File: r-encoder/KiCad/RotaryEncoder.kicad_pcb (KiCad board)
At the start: 2 copper layers, 39 x 39 mm, 15 parts, among them J1 Conn_01x06, U1 PEC11R-4325F-S0012

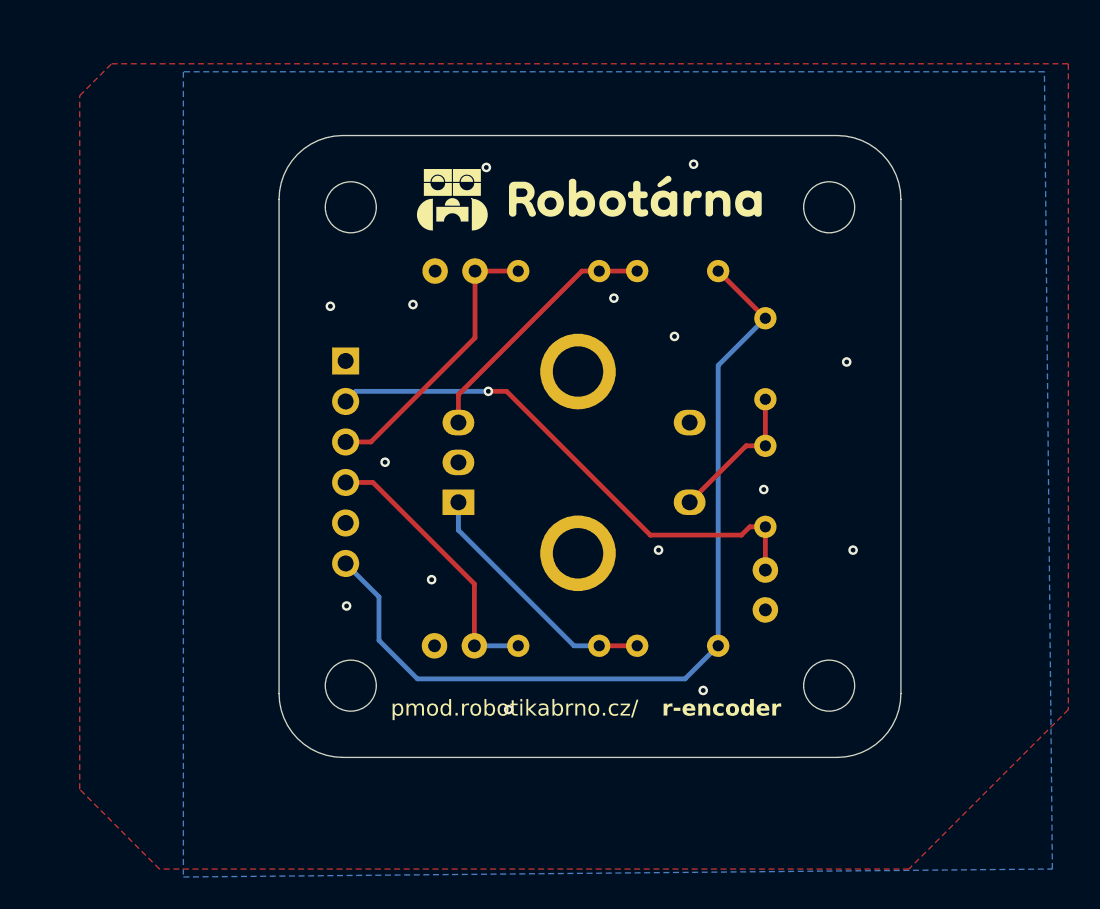
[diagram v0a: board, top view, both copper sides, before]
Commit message: Deployed d972a79 with MkDocs version: 1.6.0
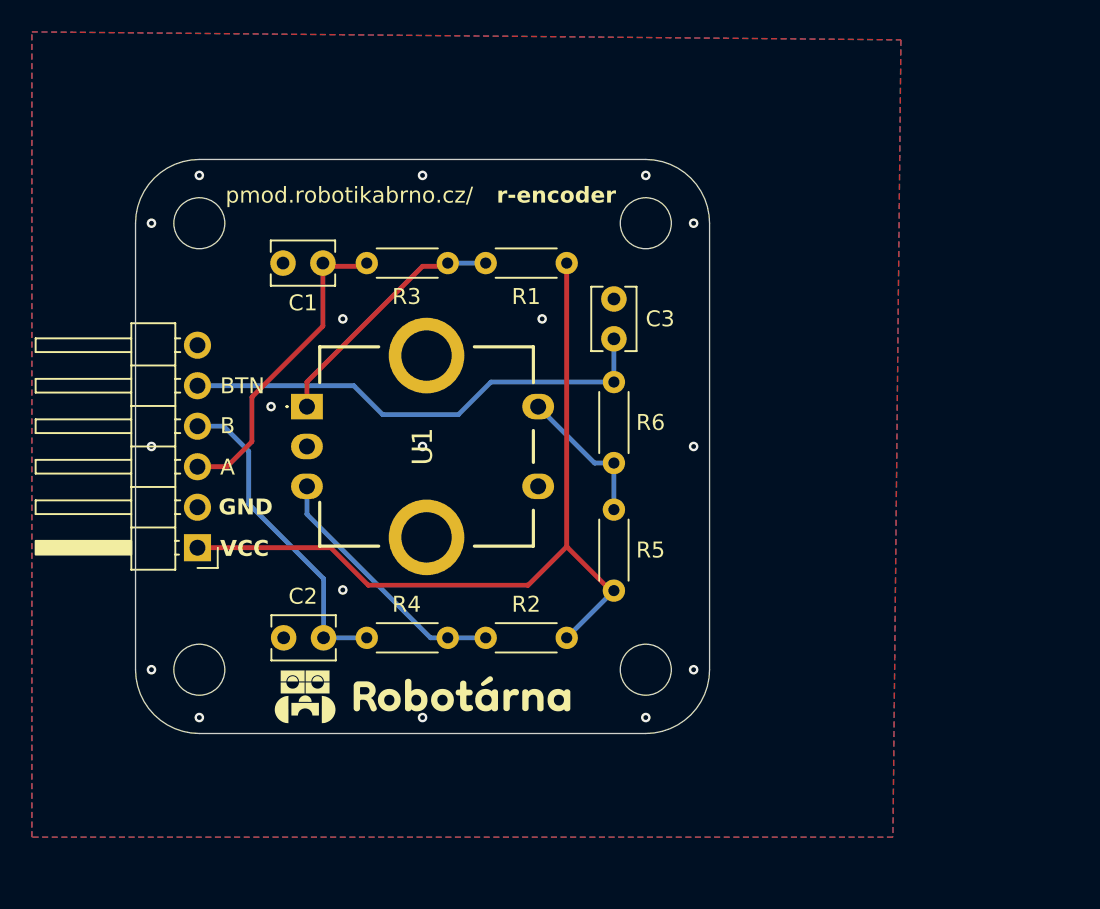
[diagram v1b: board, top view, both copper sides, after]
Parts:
- C1, C2, C3: value 0.01uF -> 10nF; moved to F.Cu
- H1, H2, H3, H4: moved to B.Cu
- J1, R1, R2, R3, R4, R5, R6, U1: moved to F.Cu
- moved H1 31.2 mm to (129.0, 99.5)
- moved H3 31.2 mm to (129.0, 71.5)
- moved H2 30.5 mm to (101.0, 99.5)
- moved H4 30.5 mm to (101.0, 71.5)
- moved C1 25.8 mm to (106.2, 74.0)
- moved R3 25.8 mm to (116.6, 74.0)
- moved R1 25.8 mm to (124.0, 74.0)
- moved C2 24.9 mm to (106.3, 97.5)
- moved R4 24.9 mm to (111.5, 97.5)
- moved R2 24.9 mm to (124.0, 97.5)
- moved C3 17.3 mm to (127.0, 78.8), turned to 90 degrees
- moved J1 15.0 mm to (100.9, 91.8)
- moved R5 11.8 mm to (127.0, 89.5), turned to -90 degrees
- moved U1 11.2 mm to (107.8, 83.0), turned to -90 degrees
- moved R6 9.56 mm to (127.0, 86.5), turned to 90 degrees
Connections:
- J1 pad 1: unconnected-(J1-Pin_1-Pad1) -> VCC
- J1 pad 2: BTN -> GND
- J1 pad 3: B -> A
- J1 pad 4: A -> B
- J1 pad 5: GND -> BTN
- J1 pad 6: VCC -> unconnected-(J1-Pin_6-Pad6)
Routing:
- net VCC: track 54.8 -> 51.1 mm
- net BTN: track 33.2 -> 30.4 mm, vias 1 -> 0
- net B: track 17.7 -> 20.5 mm
- net A: track 17.3 -> 19.9 mm
- net GND: track 0.00 -> 0.28 mm, vias 15 -> 17
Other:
- board size 39 x 39 mm -> 36 x 36 mm
- board text added: "36mm"
- board text removed: "30mm"
- board text removed: "M3"
